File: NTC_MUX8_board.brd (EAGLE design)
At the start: 76.2 x 63.5 mm, 63 parts, among them IC1 NINA-B306-00B-00, IC2 INA126E, IC3 MCP6001T_SOT23, IC4 MAX8559ETAAA+T, J1 USB4105-GF-A, J2 1761681-7, J3 DM3CS-SF-PEJMS, J4 DNP, Q1 NTR5103NT1G, U1 TMUX1208PWR, U2 TMUX1208PWR, U3 TMUX1208PWR, U4 TMUX1208PWR

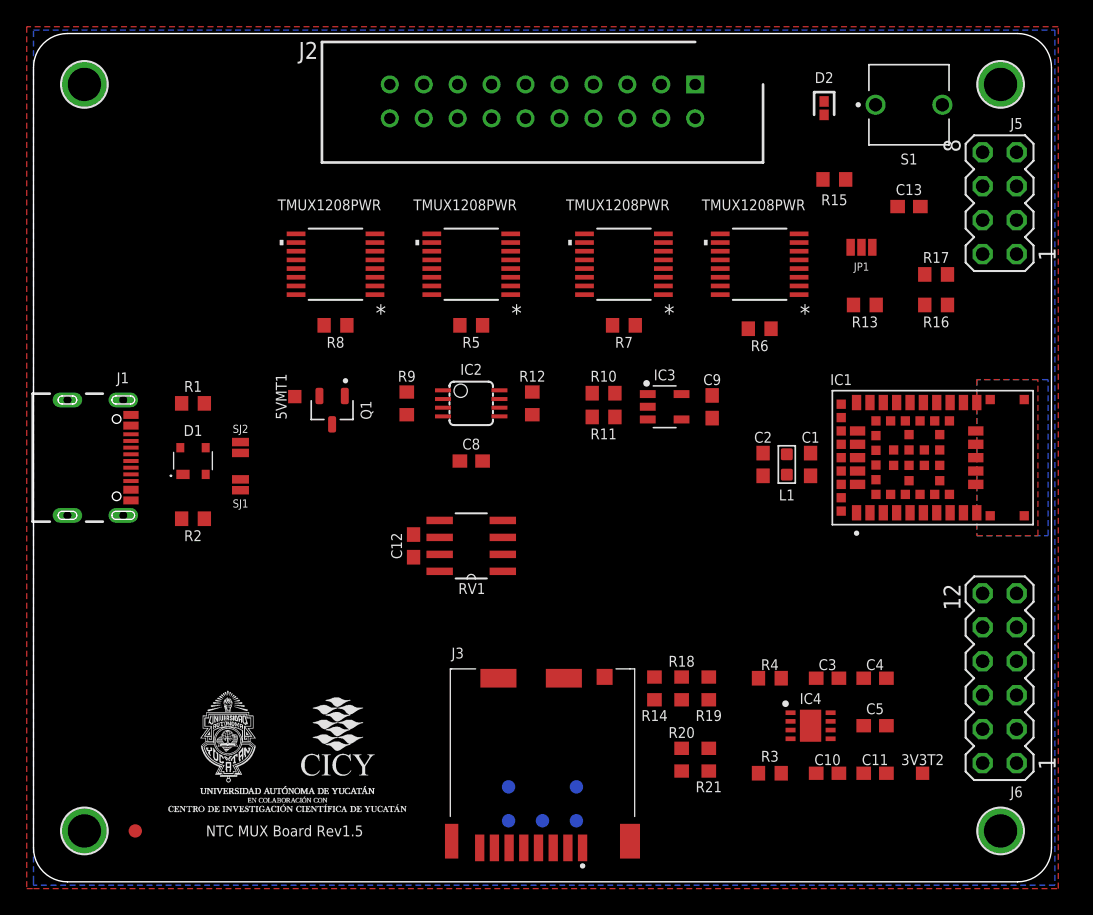
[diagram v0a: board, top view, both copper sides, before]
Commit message: Pequeños errores y adición de mejoras
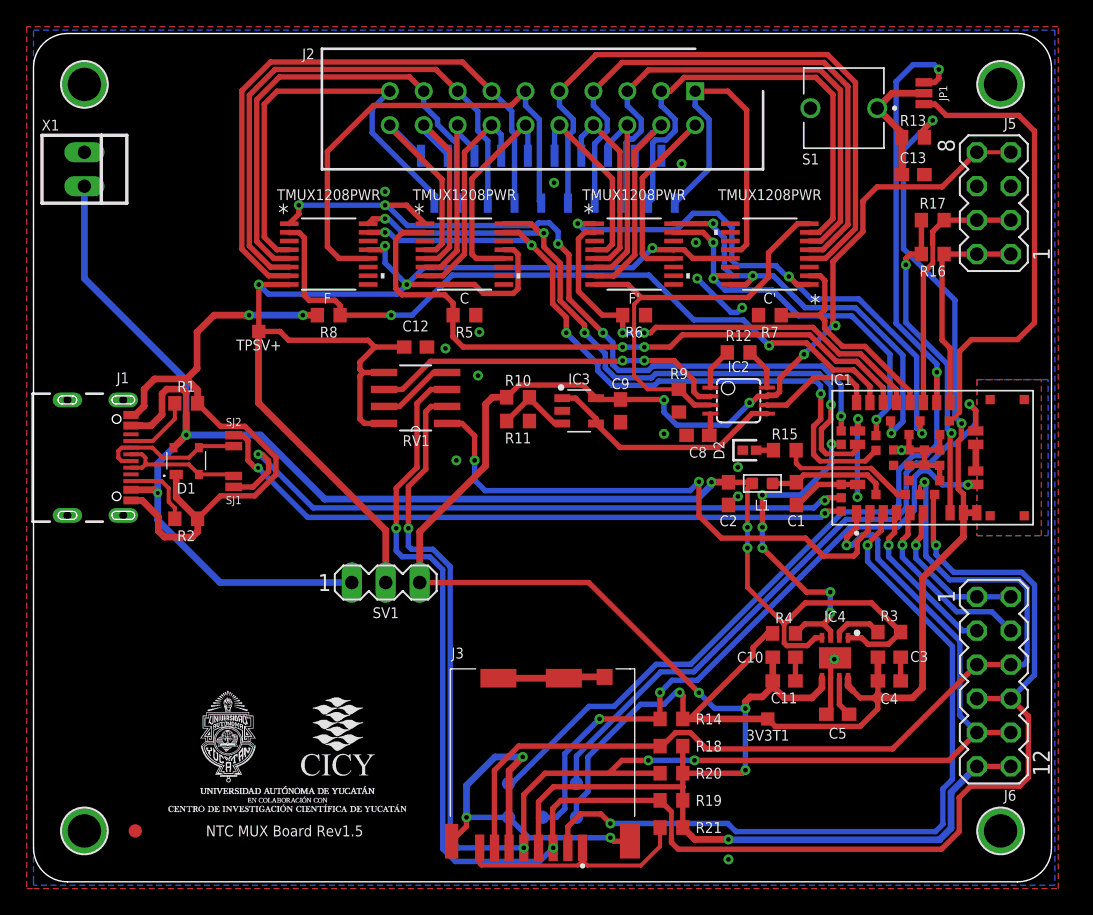
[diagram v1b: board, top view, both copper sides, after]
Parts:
- removed 3V3T2, 5VMT1: TESTPOINT_TPS-SMD-10SN, 52101-101-REV-A_v16:TESTPOINT_SMD-10SN
- removed Q1: NTR5103NT1G, NTR5103NT1G:SOT95P237X111-3N
- added 3V3T1, TPSV+: TESTPOINT_TPS-SMD-10SN, 52101-101-REV-A_v16:TESTPOINT_SMD-10SN
- added J7: 52808-2071, 52808-2071:528082071
- added SV1: (no value), con-lstb:MA03-1
- added X1: 22-23-2021, con-molex:22-23-2021
- moved D2 26.2 mm to (53.6, 32.3), turned to 0 degrees
- moved R15 20.6 mm to (56.2, 32.3)
- moved R9 20.4 mm to (48.3, 36.0)
- moved IC2 20.0 mm to (52.8, 36.0)
- moved C8 17.1 mm to (49.7, 33.4), turned to 180 degrees
- moved R12 15.9 mm to (52.8, 39.6), turned to 180 degrees
- moved C12 14.9 mm to (28.6, 40.0), turned to 0 degrees
- moved R3 13.8 mm to (64.1, 18.7), turned to 180 degrees
- moved R13 13.1 mm to (65.8, 55.7)
- moved JP1 12.4 mm to (66.6, 59.0), turned to 270 degrees
- moved RV1 11.8 mm to (28.6, 36.2)
- moved R7 10.9 mm to (55.1, 42.4)
- moved U4 10.9 mm to (55.1, 47.0)
- moved C11 9.70 mm to (56.2, 15.0), turned to 0 degrees
- moved R6 9.45 mm to (45.0, 42.4)
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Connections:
- net EN1 renamed ENI1
- net EN2 renamed ENI2
- removed net 5VMOSFET: 5VMT1.TP, C12.1, Q1.2, RV1.5, RV1.8, U1.13, U1.8, U2.13, U2.8, U3.13, U4.13
- removed net EN3: IC1.21, R6.2, U3.2
- removed net EN4: IC1.22, R7.2, U4.2
- removed net MOSFET1: Q1.1
- removed net N$13: R21.1
- new net DAT: J3.1, J3.8, R21.1
- new net ENO1: IC1.22, R6.2, U3.2
- new net ENO2: IC1.21, R7.2, U4.2
- new net VSEL: C12.1, RV1.5, RV1.8, SV1.2, TPSV+.TP, U1.13, U1.8, U2.13, U2.8, U3.13, U4.13
- net 3V3_1: now also 3V3T1.TP
- net 3V3_2: now also SV1.3; no longer 3V3T2.TP
- net AIN0: now also IC1.49
- net AIN1: now also IC1.27
- net AIN2: now also IC1.44
- net AOUT0: now also IC1.39
- net AOUT1: now also IC1.41
- net AOUT2: now also IC1.43
- net C1IN: now also J2.20, J7.20, U2.4; no longer J2.19, U1.11
- net C1OUT: now also J2.9, J7.9, U4.4; no longer J2.10, U3.11
- net C2IN: now also J2.18, J7.18, U2.5; no longer J2.17, U1.10
- net C2OUT: now also J2.7, J7.7, U4.5; no longer J2.8, U3.10
- net C3IN: now also J2.16, J7.16, U2.6; no longer J2.15, U1.9
- net C3OUT: now also J2.5, J7.5, U4.6; no longer J2.6, U3.9
- net C4IN: now also J2.14, J7.14, U2.7; no longer J2.13, U2.4
- net C4OUT: now also J2.3, J7.3, U4.7; no longer J2.4, U4.4
- net C5IN: now also J2.12, J7.12, U2.12; no longer J2.11, U2.5
- net C5OUT: now also J2.1, J7.1, U4.12; no longer J2.2, U4.5
- net CS_3: now also J6.3; no longer J6.4
- net CS_4: now also J6.4; no longer J6.3
- net F1IN: now also J2.19, J7.19; no longer J2.20
- net F1OUT: now also J2.10, J7.10; no longer J2.9
- net F2IN: now also J2.17, J7.17; no longer J2.18
- net F2OUT: now also J2.8, J7.8; no longer J2.7
- net F3IN: now also J2.15, J7.15; no longer J2.16
- net F3OUT: now also J2.6, J7.6; no longer J2.5
- net F4IN: now also J2.13, J7.13; no longer J2.14
- net F4OUT: now also J2.4, J7.4; no longer J2.3
- net F5IN: now also J2.11, J7.11; no longer J2.12
- net F5OUT: now also J2.2, J7.2; no longer J2.1
- net GND: now also X1.1
- net GP_PB: now also IC1.37
- net VBUS: no longer Q1.3
- net V_EN: now also IC1.50; no longer IC1.49
- net V_USB: now also SV1.1, X1.2
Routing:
- net 3V3_2: track 0.00 -> 168.2 mm, vias 0 -> 8
- net GND: track 0.00 -> 142.6 mm, vias 0 -> 24
- net V_USB: track 0.00 -> 134.6 mm, vias 0 -> 5
- net SPI_MOSI: track 0.00 -> 125.0 mm, vias 0 -> 3
- net SPI_SCK: track 0.00 -> 111.6 mm, vias 0 -> 5
- net VSEL: track 0.00 -> 104.3 mm, vias 0 -> 4
- net 3V3_1: track 0.00 -> 101.0 mm, vias 0 -> 3
- net RESETN: track 0.00 -> 80.6 mm, vias 0 -> 2
- net SPI_MISO: track 0.00 -> 70.8 mm, vias 0 -> 1
- net AIN0: track 0.00 -> 58.7 mm, vias 0 -> 5
- net SD_CS: track 0.00 -> 57.6 mm, vias 0 -> 2
- net AIN1: track 0.00 -> 55.1 mm, vias 0 -> 4
- net ENI1: track 0.00 -> 55.1 mm, vias 0 -> 2
- net AIN2: track 0.00 -> 54.6 mm, vias 0 -> 4
- net USB_P: track 0.00 -> 50.5 mm, vias 0 -> 2
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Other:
- board text added: "C"
- board text added: "C'"
- board text added: "F"
- board text added: "F'"
